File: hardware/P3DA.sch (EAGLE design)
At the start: 70 parts, among them J2 22-27-2041-04, J3 22-27-2041-04, J4 22-27-2041-04, J5 22-27-2041-04, J6 22-27-2041-04, J7 22-27-2041-04, X7 9090-4R

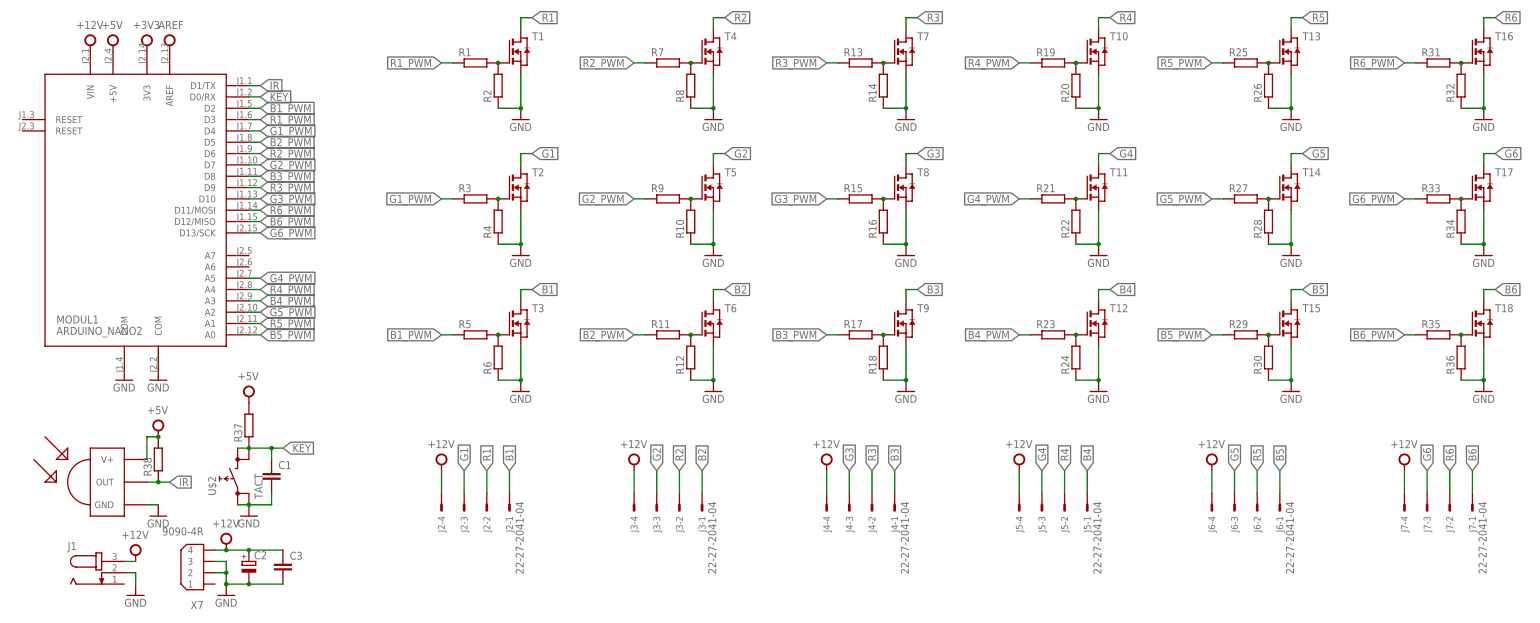
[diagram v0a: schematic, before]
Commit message: Refactoring PCB and schematic
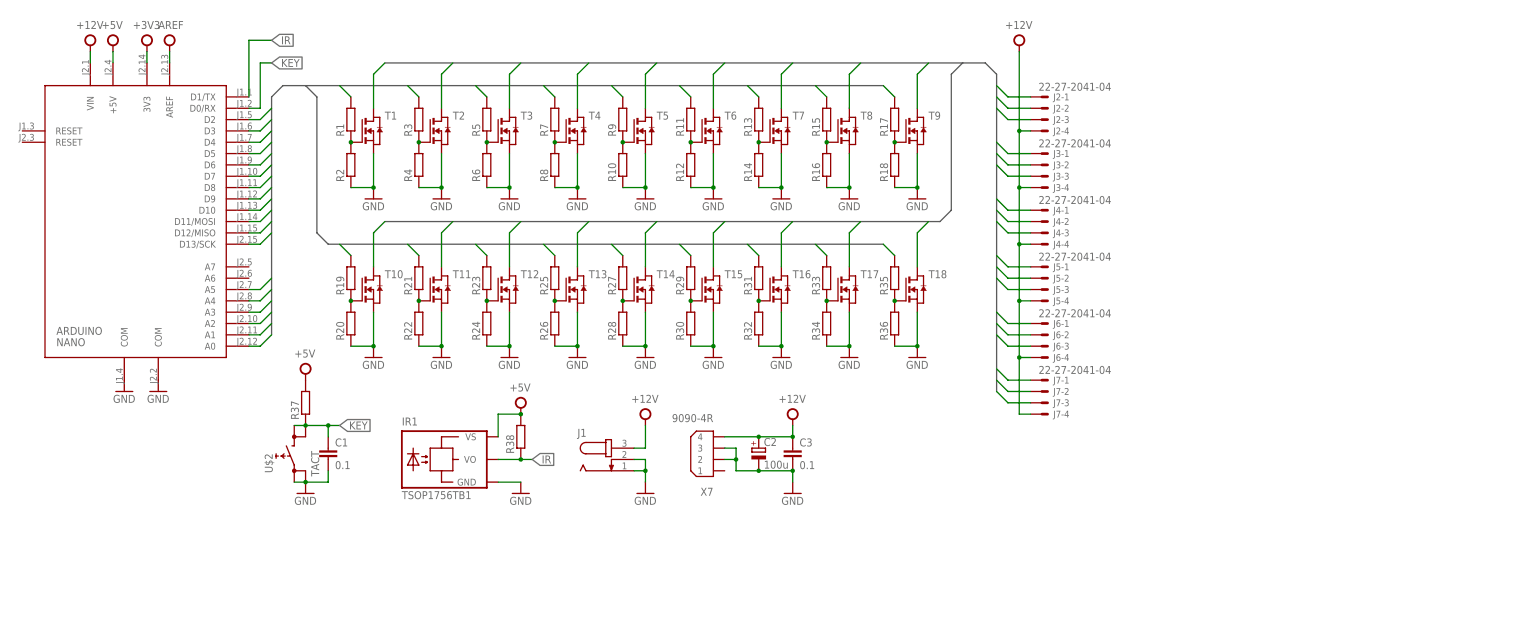
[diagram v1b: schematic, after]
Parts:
- removed MODUL1: ARDUINO_NANO2, arduino:ARDUINO_NANO2
- removed U$1: TSOP1738, tsop:TSOP1738
- added ARDUINO: NANO, arduino:ARDUINO_NANO2
- added IR1: TSOP1756TB1, telefunken:TSOP1756TB1
- C1, C3: value (none) -> 0.1
- C2: value (none) -> 100u
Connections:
- removed net B1_PWM: MODUL1.D2, R5.1
- removed net B2_PWM: MODUL1.D5, R11.1
- removed net B3_PWM: MODUL1.D8, R17.1
- removed net B4_PWM: MODUL1.A3, R23.1
- removed net B5_PWM: MODUL1.A0, R29.1
- removed net B6_PWM: MODUL1.D12/MISO, R35.1
- removed net G1_PWM: MODUL1.D4, R3.1
- removed net G2_PWM: MODUL1.D7, R9.1
- removed net G3_PWM: MODUL1.D10, R15.1
- removed net G4_PWM: MODUL1.A5, R21.1
- removed net G5_PWM: MODUL1.A2, R27.1
- removed net G6_PWM: MODUL1.D13/SCK, R33.1
- removed net N$1: R1.2, R2.2, T1.G
- removed net N$4: R3.2, R4.2, T2.G
- removed net R1_PWM: MODUL1.D3, R1.1
- removed net R2_PWM: MODUL1.D6, R7.1
- removed net R3_PWM: MODUL1.D9, R13.1
- removed net R4_PWM: MODUL1.A4, R19.1
- removed net R5_PWM: MODUL1.A1, R25.1
- removed net R6_PWM: MODUL1.D11/MOSI, R31.1
- new net B_IN1: ARDUINO.D2, R5.2
- new net B_IN2: ARDUINO.D5, R11.2
- new net B_IN3: ARDUINO.D8, R17.2
- new net B_IN4: ARDUINO.A3, R23.2
- new net B_IN5: ARDUINO.A0, R29.2
- new net B_IN6: ARDUINO.D12/MISO, R35.2
- new net G_IN1: ARDUINO.D4, R3.2
- new net G_IN2: ARDUINO.D7, R9.2
- new net G_IN3: ARDUINO.D10, R15.2
- new net G_IN4: ARDUINO.A5, R21.2
- new net G_IN5: ARDUINO.A2, R27.2
- new net G_IN6: ARDUINO.D13/SCK, R33.2
- new net N$19: R1.1, R2.2, T1.G
- new net N$20: R3.1, R4.2, T2.G
- new net R_IN1: ARDUINO.D3, R1.2
- new net R_IN2: ARDUINO.D6, R7.2
- new net R_IN3: ARDUINO.D9, R13.2
- new net R_IN4: ARDUINO.A4, R19.2
- new net R_IN5: ARDUINO.A1, R25.2
- new net R_IN6: ARDUINO.D11/MOSI, R31.2
- net +12V: now also ARDUINO.VIN; no longer MODUL1.VIN
- net +3V3: now also ARDUINO.3V3; no longer MODUL1.3V3
- net +5V: now also ARDUINO.+5V, IR1.VS; no longer MODUL1.+5V, U$1.V+
- net AREF: now also ARDUINO.AREF; no longer MODUL1.AREF
- net GND: now also ARDUINO.COM, ARDUINO.COM@1, IR1.GND, J1.1; no longer MODUL1.COM, MODUL1.COM@1, U$1.GND
- net IR: now also ARDUINO.D1/TX, IR1.VO; no longer MODUL1.D1/TX, U$1.OUT
- net KEY: now also ARDUINO.D0/RX; no longer MODUL1.D0/RX
- net N$10: now also R19.1; no longer R19.2
- net N$11: now also R21.1; no longer R21.2
- net N$12: now also R23.1; no longer R23.2
- net N$13: now also R25.1; no longer R25.2
- net N$14: now also R27.1; no longer R27.2
- net N$15: now also R29.1; no longer R29.2
- net N$16: now also R31.1; no longer R31.2
- net N$17: now also R33.1; no longer R33.2
- net N$18: now also R35.1; no longer R35.2
- net N$2: now also R7.1; no longer R7.2
- net N$3: now also R9.1; no longer R9.2
- net N$5: now also R5.1; no longer R5.2
- net N$6: now also R11.1; no longer R11.2
- net N$7: now also R13.1; no longer R13.2
- net N$8: now also R15.1; no longer R15.2
- net N$9: now also R17.1; no longer R17.2
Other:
- moved on the sheet: C1, C2, C3, J1, J2-1, J2-2, J2-3, J2-4, J3-1, J3-2, J3-3, J3-4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
